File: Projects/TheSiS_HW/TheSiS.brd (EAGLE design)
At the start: 92.7 x 98.7 mm, 80 parts, among them IC1 REG1117, IC3 TP4056, IC4 MCP1703CB, IC5 CP2102, K1 G5L, K2 G5L, K3 G5L, T1 DMN3024LSD, U1 ESP-WROOM-32, U2 GY-521MPU6050, X2 ZX62D-B-5PA8

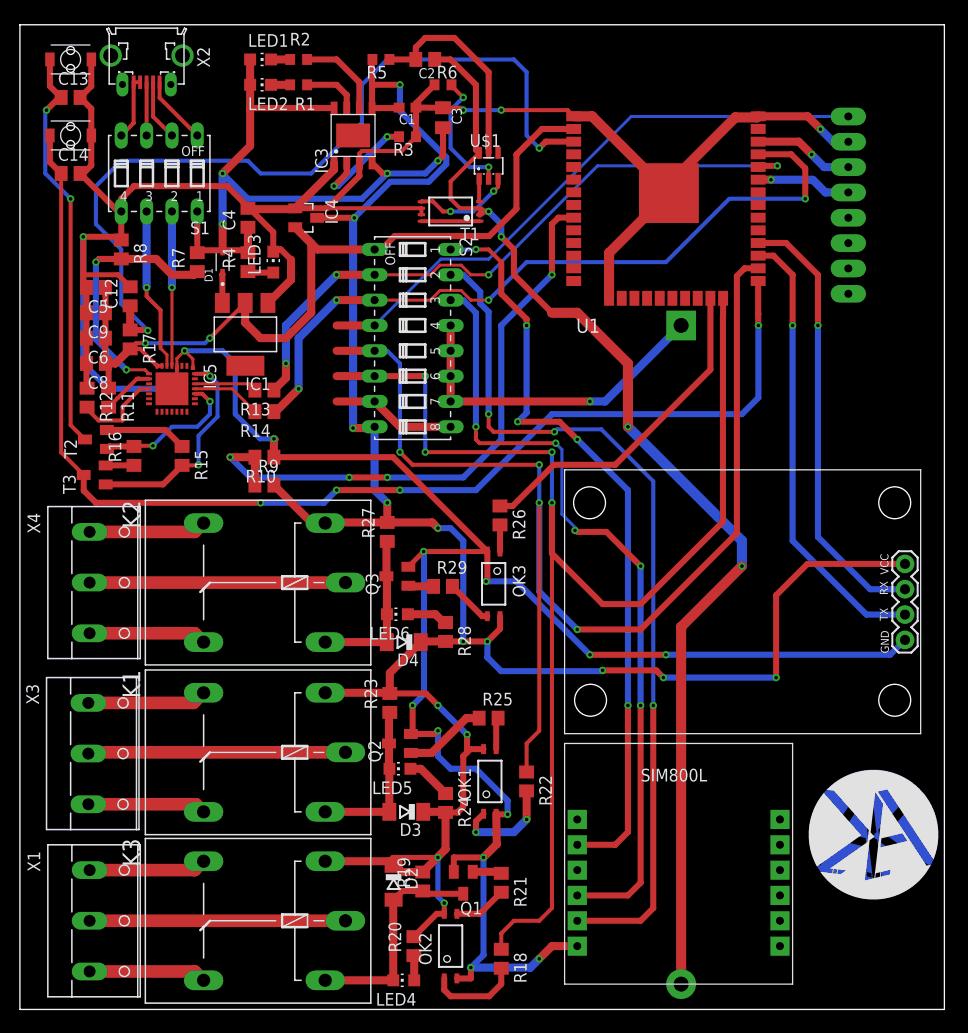
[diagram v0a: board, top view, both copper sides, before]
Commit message: Finish Hardware v20.10.21
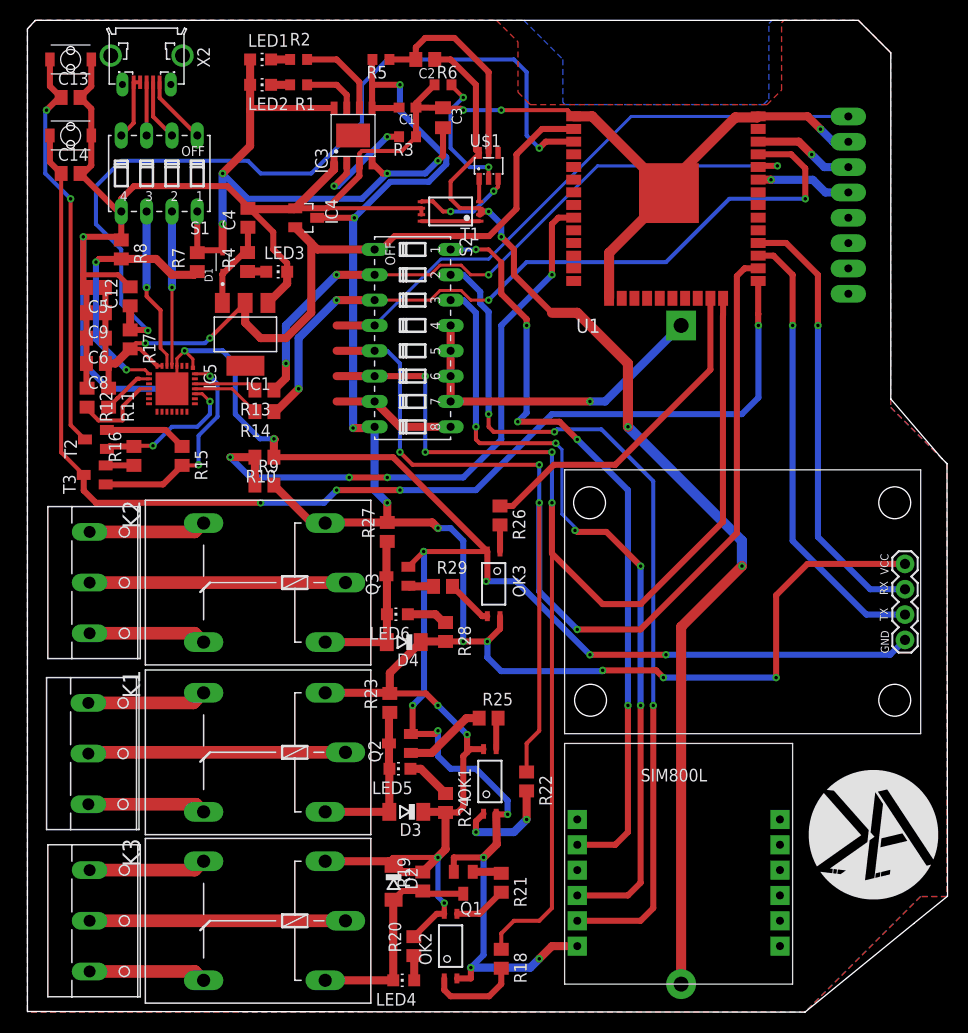
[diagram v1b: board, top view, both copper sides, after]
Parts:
- moved LED3 1.02 mm to (63.0, 87.6), turned to 270 degrees
- renumbered U$2 to 18650
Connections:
- new net EXT5V: C4.1, D1.C, IC1.3, R4.2
- net VIN5V: no longer C4.1, D1.C, IC1.3, R4.2
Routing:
- net EXT5V: track 0.00 -> 8.85 mm
- net VIN5V: track 73.4 -> 65.3 mm
- net GND: track 382.4 -> 381.5 mm
- net N$10: track 2.58 -> 1.88 mm
- added copper zone on layer 1, net GND
- added copper zone on layer 16, net GND
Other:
- board size 92.7 x 98.7 mm -> 92.3 x 99.4 mm

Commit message: Finish Board v20.10.20 [Order PCBWay.com]
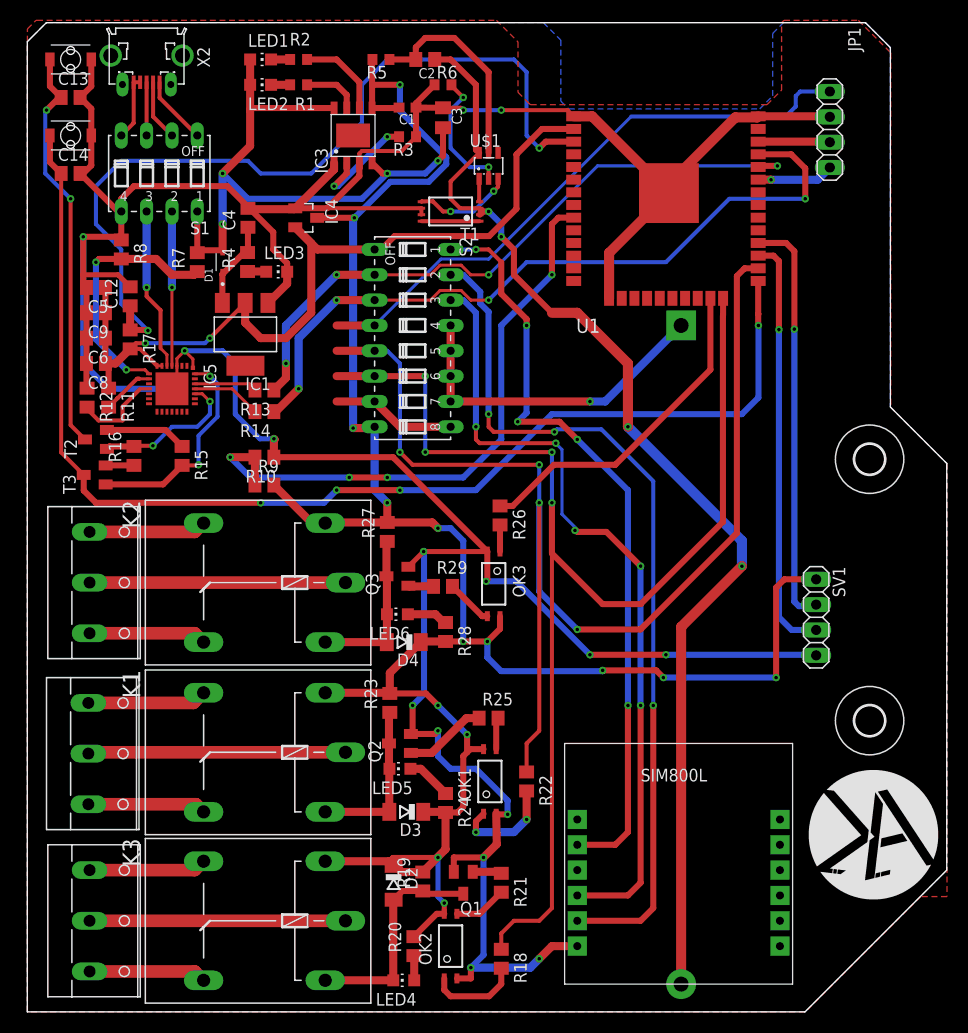
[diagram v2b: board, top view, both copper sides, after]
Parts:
- removed U2: GY-521MPU6050, gy-521:GY-521
- added JP1, SV1: (no value), pinhead:1X04
- added U$2: (no value), holes:3,0
- U$3: value U-BLOX-NEO6V2 -> (none); device u-blox neo-6m v2:U-BLOX-NEO6V2 -> holes:3,0
- moved U$3 39.6 mm to (122.4, 42.5), turned to 0 degrees
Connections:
- removed net N$33: S2.4, U2.VCC
- removed net N$37: U2.XDA
- removed net N$38: U2.XCL
- removed net N$39: U2.ADO
- removed net N$40: U2.INT
- new net N$35: JP1.1, S2.4
- net BAT+: now also SV1.1; no longer U$3.VCC
- net GND: now also JP1.2, SV1.4; no longer U$3.GND, U2.GND
- net IO16: now also SV1.3; no longer U$3.TX
- net IO17: now also SV1.2; no longer U$3.RX
- net IO21: now also JP1.4; no longer U2.SDA
- net IO22: now also JP1.3; no longer U2.SCL
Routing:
- net N$33: track 60.0 -> 0.00 mm
- net N$35: track 0.00 -> 59.8 mm
- net GND: track 381.5 -> 369.1 mm, vias 16 -> 15
- net BAT+: track 232.1 -> 223.0 mm
- net IO16: track 45.2 -> 42.3 mm
- net IO17: track 44.5 -> 41.5 mm
- net IO22: track 10.1 -> 7.21 mm, vias 1 -> 0
- net IO21: track 9.57 -> 7.70 mm
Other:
- board size 92.3 x 99.4 mm -> 92.2 x 99.2 mm
